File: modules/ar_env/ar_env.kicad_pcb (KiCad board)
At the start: 2 copper layers, 30.5 x 68.6 mm, 4 parts

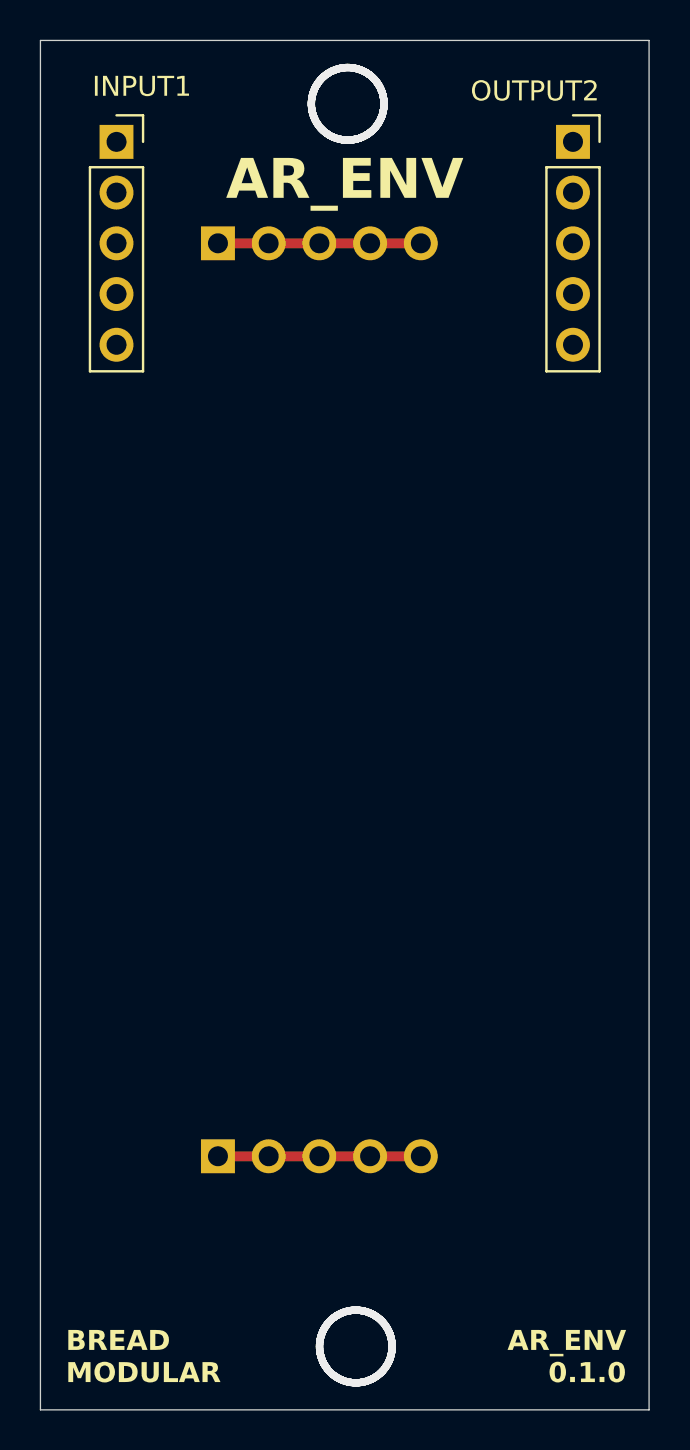
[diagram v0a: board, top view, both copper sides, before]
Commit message: Finalize the PCB
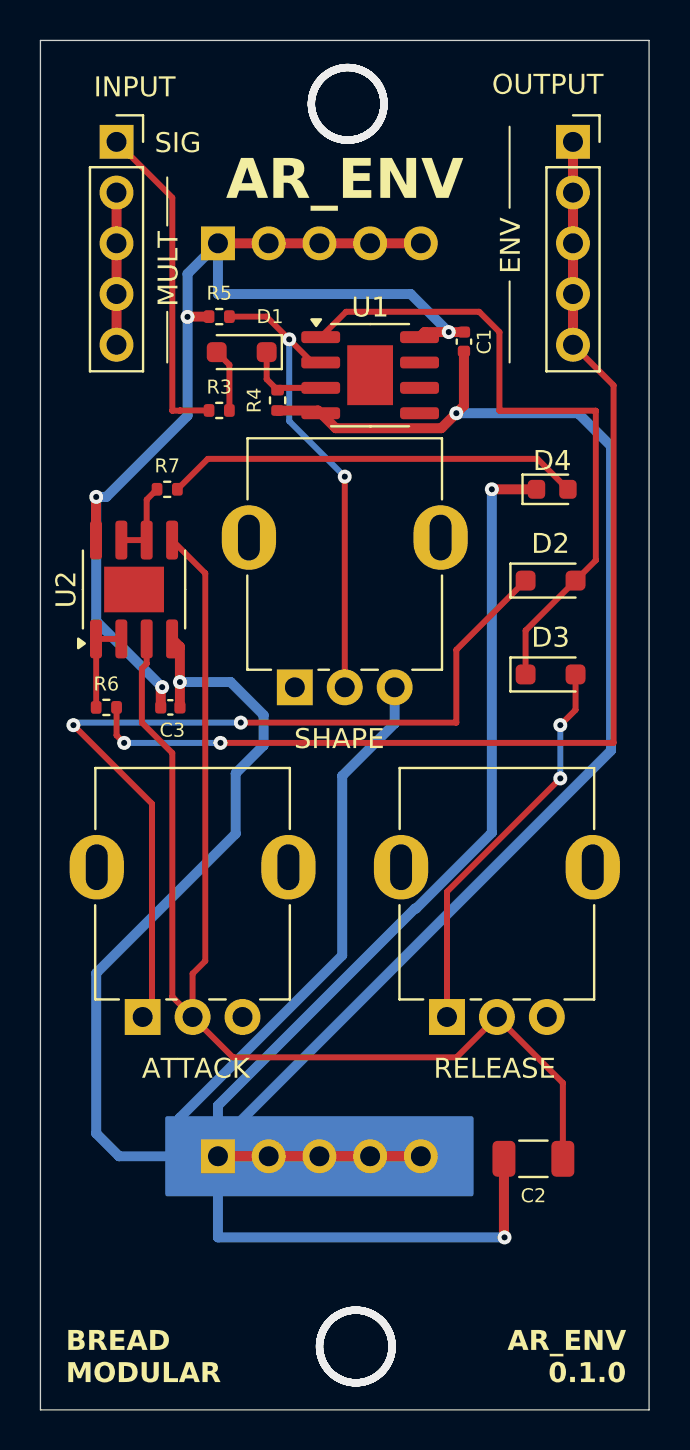
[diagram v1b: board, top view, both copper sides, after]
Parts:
- added C1: 0.1uf, Capacitor_SMD:C_0402_1005Metric, F.Cu at (68.2, 55.7)
- added C2: 1uf, Capacitor_SMD:C_1206_3216Metric, F.Cu at (71.7, 96.6)
- added C3: 0.1uf, Capacitor_SMD:C_0402_1005Metric, F.Cu at (53.5, 74.0)
- added D1: 1N4148WS, Diode_SMD:D_SOD-323_HandSoldering, F.Cu at (57.1, 56.2)
- added D2: 1N4148WS, Diode_SMD:D_SOD-323_HandSoldering, F.Cu at (72.5, 67.7)
- added D3: 1N4148WS, Diode_SMD:D_SOD-323_HandSoldering, F.Cu at (72.5, 72.4)
- added D4: LED, LED_SMD:LED_0603_1608Metric, F.Cu at (72.6, 63.1)
- added R3: 100k, Resistor_SMD:R_0402_1005Metric, F.Cu at (55.9, 59.2)
- added R4: 100k, Resistor_SMD:R_0402_1005Metric, F.Cu at (58.9, 58.7)
- added R5: 6.8k, Resistor_SMD:R_0402_1005Metric, F.Cu at (55.9, 54.5)
- added R6: 1k, Resistor_SMD:R_0402_1005Metric, F.Cu at (50.3, 74.0)
- added R7: 1k, Resistor_SMD:R_0402_1005Metric, F.Cu at (53.3, 63.1)
- added RV1: 5k, BreadModular_Pots:Potentiometer_RV09, F.Cu at (59.7, 73.0)
- added RV2: 1M, BreadModular_Pots:Potentiometer_RV09, F.Cu at (52.1, 89.5)
- added RV3: 1M, BreadModular_Pots:Potentiometer_RV09, F.Cu at (67.3, 89.5)
- added U1: MCP6002-xSN, Package_SO:SOIC-8-1EP_3.9x4.9mm_P1.27mm_EP2.29x3mm, F.Cu at (63.5, 57.4)
- added U2: MCP6002-xSN, Package_SO:SOIC-8-1EP_3.9x4.9mm_P1.27mm_EP2.29x3mm, F.Cu at (51.7, 68.1)
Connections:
- INPUT1 pad 1: unconnected-(INPUT1-Pin_1-Pad1) -> V_IN
- INPUT1 pad 2: unconnected-(INPUT1-Pin_2-Pad2) -> Net-(INPUT1-Pin_2)
- INPUT1 pad 3: unconnected-(INPUT1-Pin_3-Pad3) -> Net-(INPUT1-Pin_2)
- INPUT1 pad 4: unconnected-(INPUT1-Pin_4-Pad4) -> Net-(INPUT1-Pin_2)
- INPUT1 pad 5: unconnected-(INPUT1-Pin_5-Pad5) -> Net-(INPUT1-Pin_2)
- OUTPUT2 pad 1: unconnected-(OUTPUT2-Pin_1-Pad1) -> V_OUT
- OUTPUT2 pad 2: unconnected-(OUTPUT2-Pin_2-Pad2) -> V_OUT
- OUTPUT2 pad 3: unconnected-(OUTPUT2-Pin_3-Pad3) -> V_OUT
- OUTPUT2 pad 4: unconnected-(OUTPUT2-Pin_4-Pad4) -> V_OUT
- OUTPUT2 pad 5: unconnected-(OUTPUT2-Pin_5-Pad5) -> V_OUT
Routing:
- net GND: track 10.2 -> 207.1 mm, vias 0 -> 4
- net V_SHAPE: track 0.00 -> 70.3 mm
- net V_OUT: track 0.00 -> 57.4 mm, vias 0 -> 2
- net +5V: track 10.2 -> 58.1 mm, vias 0 -> 4
- net Net-(D2-K): track 0.00 -> 44.2 mm, vias 0 -> 2
- net Net-(D2-A): track 0.00 -> 33.3 mm
- net Net-(U1A--): track 0.00 -> 24.1 mm, vias 0 -> 2
- net Net-(D4-A): track 0.00 -> 20.8 mm
- net Net-(D3-A): track 0.00 -> 19.8 mm, vias 0 -> 2
- net V_IN: track 0.00 -> 16.5 mm
- net Net-(INPUT1-Pin_2): track 0.00 -> 7.62 mm
- net Net-(U2A--): track 0.00 -> 4.70 mm
- net Net-(D1-K): track 0.00 -> 4.34 mm
- net Net-(U2B--): track 0.00 -> 4.03 mm
- net Net-(D1-A): track 0.00 -> 3.18 mm
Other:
- board text added: "ATTACK"
- board text added: "ENV"
- board text added: "INPUT"
- board text added: "MULT"
- board text added: "OUTPUT"
- board text added: "RELEASE"
- board text added: "SHAPE"
- board text added: "SIG"
